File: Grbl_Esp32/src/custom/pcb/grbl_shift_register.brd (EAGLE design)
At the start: 75 parts

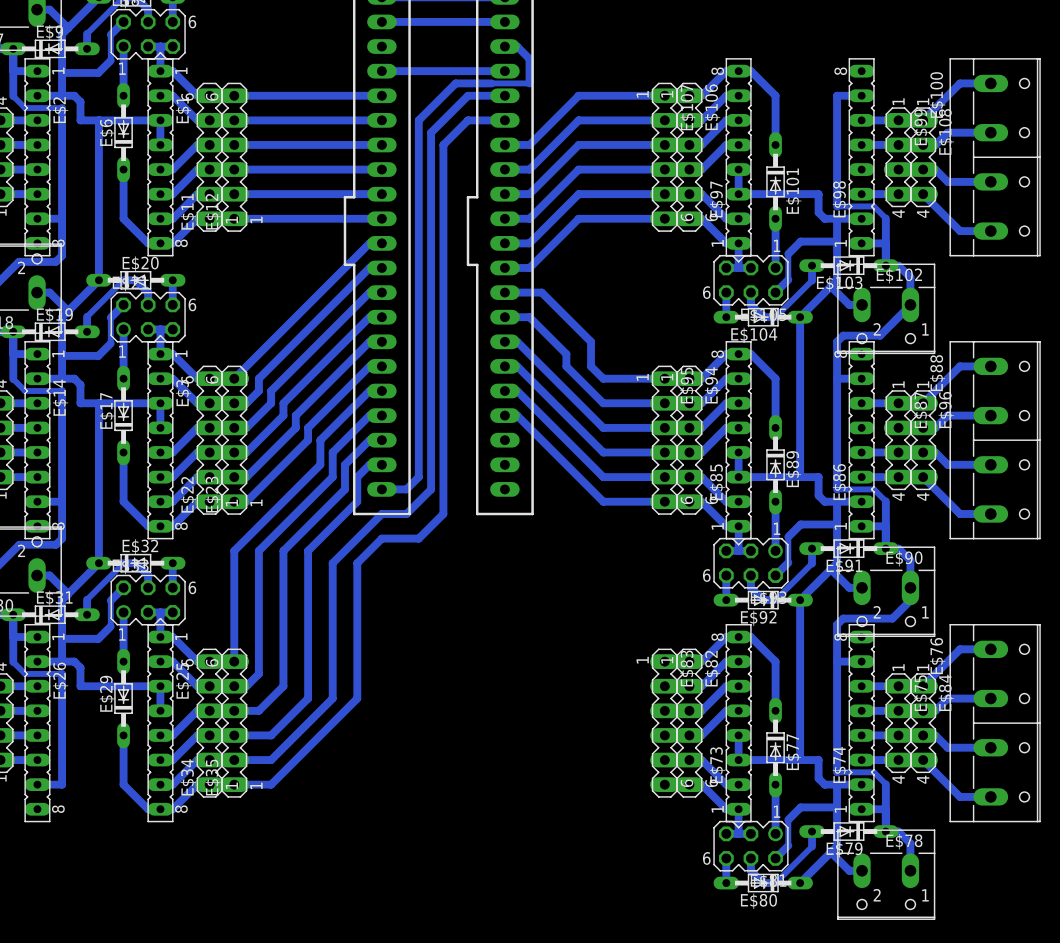
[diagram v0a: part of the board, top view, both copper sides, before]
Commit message: pcb
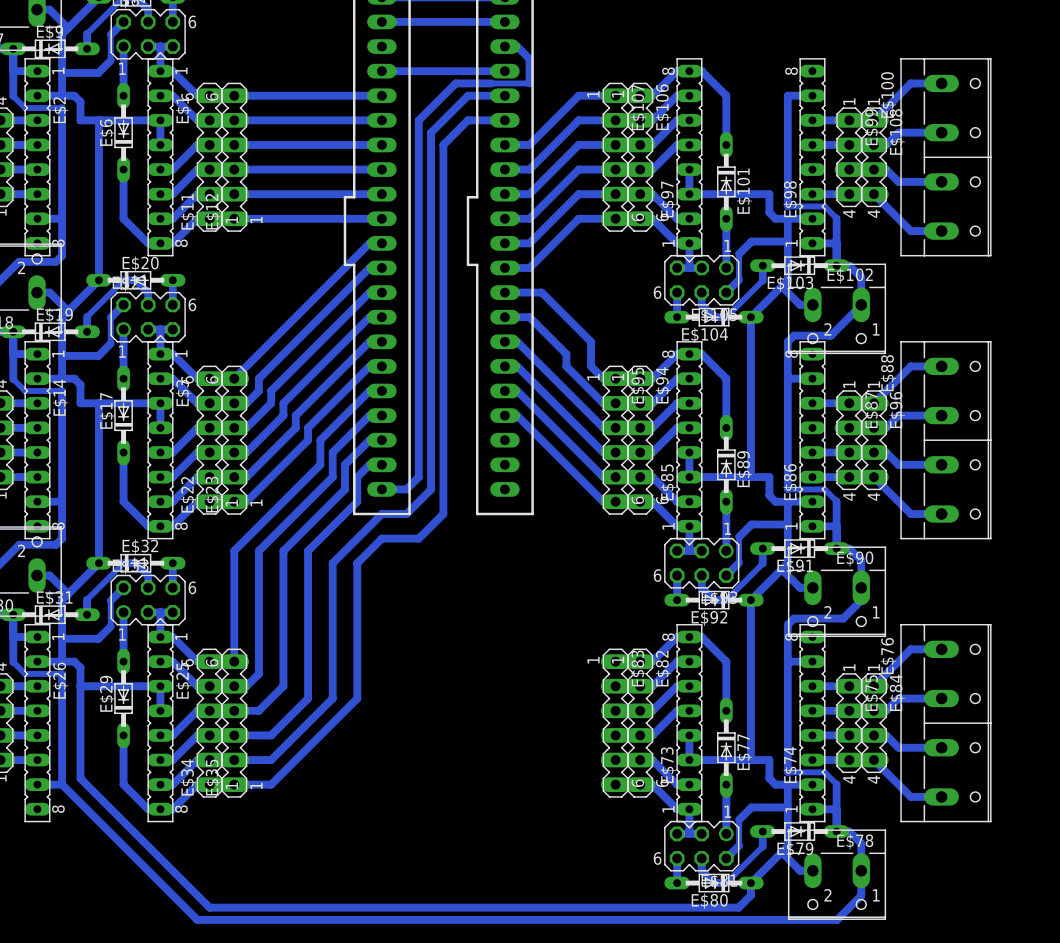
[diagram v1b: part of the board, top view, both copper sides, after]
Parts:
- moved E$75 5.08 mm to (101.6, 16.5)
- moved E$87 5.08 mm to (101.6, 45.7)
- moved E$99 5.08 mm to (101.6, 74.9)
- moved E$100 5.08 mm to (111.8, 74.9)
- moved E$101 5.08 mm to (88.9, 72.4)
- moved E$102 5.08 mm to (100.3, 58.4)
- moved E$103 5.08 mm to (96.5, 63.7)
- moved E$104 5.08 mm to (87.6, 58.4)
- moved E$105 5.08 mm to (86.4, 62.2)
- moved E$106 5.08 mm to (80.0, 74.9)
- moved E$107 5.08 mm to (77.5, 74.9)
- moved E$108 5.08 mm to (104.1, 74.9)
- moved E$73 5.08 mm to (85.1, 16.5)
- moved E$74 5.08 mm to (97.8, 16.5)
- moved E$76 5.08 mm to (111.8, 16.5)
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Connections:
- removed net S$83: E$102.1, E$103.C, E$74.1, E$74.7, E$78.1, E$79.C, E$86.1, E$86.7, E$90.1, E$91.C, E$98.1, E$98.7
- removed net S$84: E$102.2, E$104.C, E$105.2, E$73.3, E$73.4, E$74.2, E$78.2, E$80.C, E$81.2, E$85.3, E$85.4, E$86.2, E$90.2, E$92.C, E$93.2, E$97.3, E$97.4, E$98.2
- net S$6: now also E$102.2, E$104.C, E$105.2, E$73.3, E$73.4, E$74.2, E$78.2, E$80.C, E$81.2, E$85.3, E$85.4, E$86.2, E$90.2, E$92.C, E$93.2, E$97.3, E$97.4, E$98.2
- net S$60: now also E$102.1, E$103.C, E$74.1, E$74.7, E$78.1, E$79.C, E$86.1, E$86.7, E$90.1, E$91.C, E$98.1, E$98.7
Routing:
- net S$6: track 163.0 -> 412.0 mm
- net S$60: track 131.2 -> 355.1 mm
- net S$84: track 163.0 -> 0.00 mm
- net S$83: track 132.0 -> 0.00 mm
- net S$115: track 37.2 -> 32.1 mm
- net S$102: track 40.3 -> 35.2 mm
- net S$123: track 27.3 -> 22.2 mm
- net S$122: track 27.3 -> 22.2 mm
- net S$121: track 27.3 -> 22.2 mm
- net S$120: track 27.3 -> 22.2 mm
- net S$110: track 28.9 -> 23.8 mm
- net S$108: track 28.9 -> 23.8 mm
- net S$109: track 29.6 -> 24.5 mm
- net S$107: track 28.9 -> 23.8 mm
- net S$116: track 32.4 -> 27.3 mm
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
